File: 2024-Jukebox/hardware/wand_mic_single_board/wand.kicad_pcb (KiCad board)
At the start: 4 copper layers, 17.5 x 39 mm, 50 parts, among them J1 USB_C_Receptacle_USB2.0, J10 Conn_01x03, J4 Conn_01x02, J6 Conn_01x01, J9 Conn_01x02, Q1 MUN5214DW1T1G, Q3 CJ3139K, U1 CP2104, U2 ESP32-PICO-D4, U3 ICM-20948, U4 TP4065-4.2V, U5 TLV76718DRVx, U6 LY68L6400SLIT, U7 PCA9306, U9 TLV76733DRVx

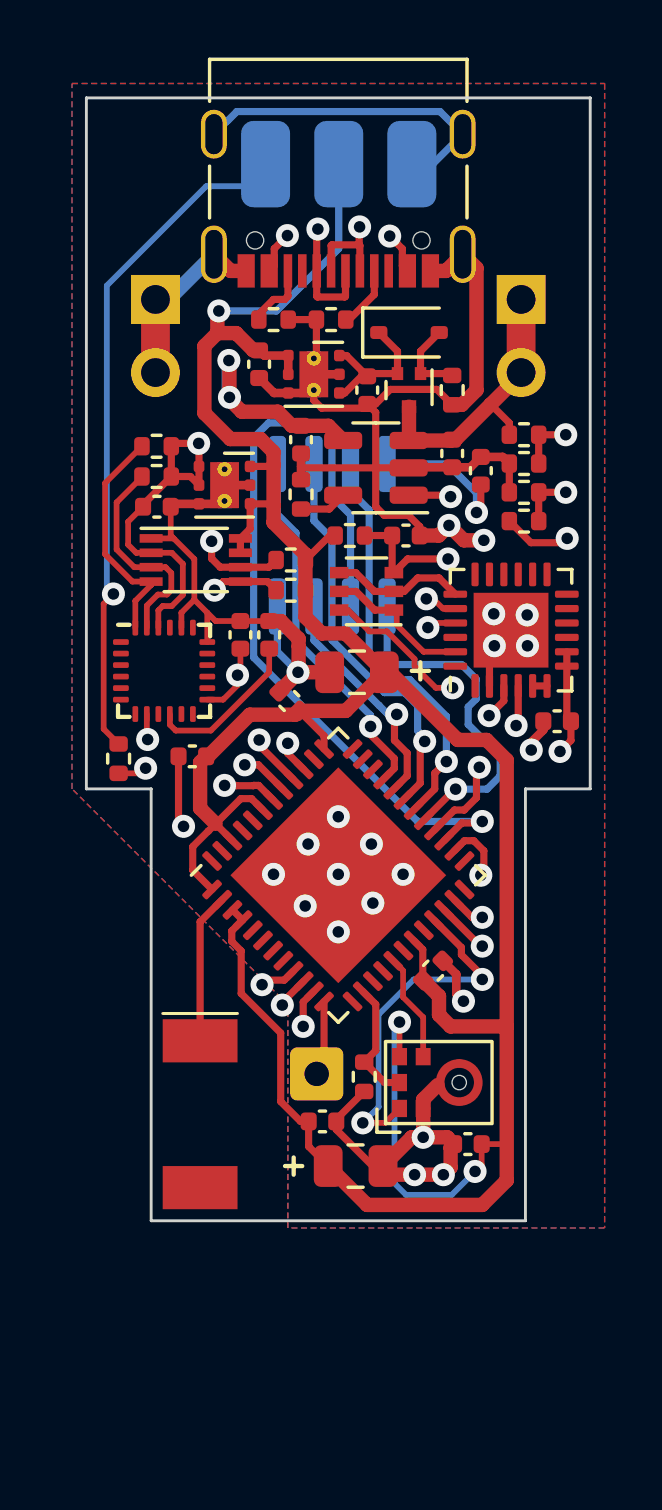
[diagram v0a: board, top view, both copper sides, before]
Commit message: Updated wand PCBs
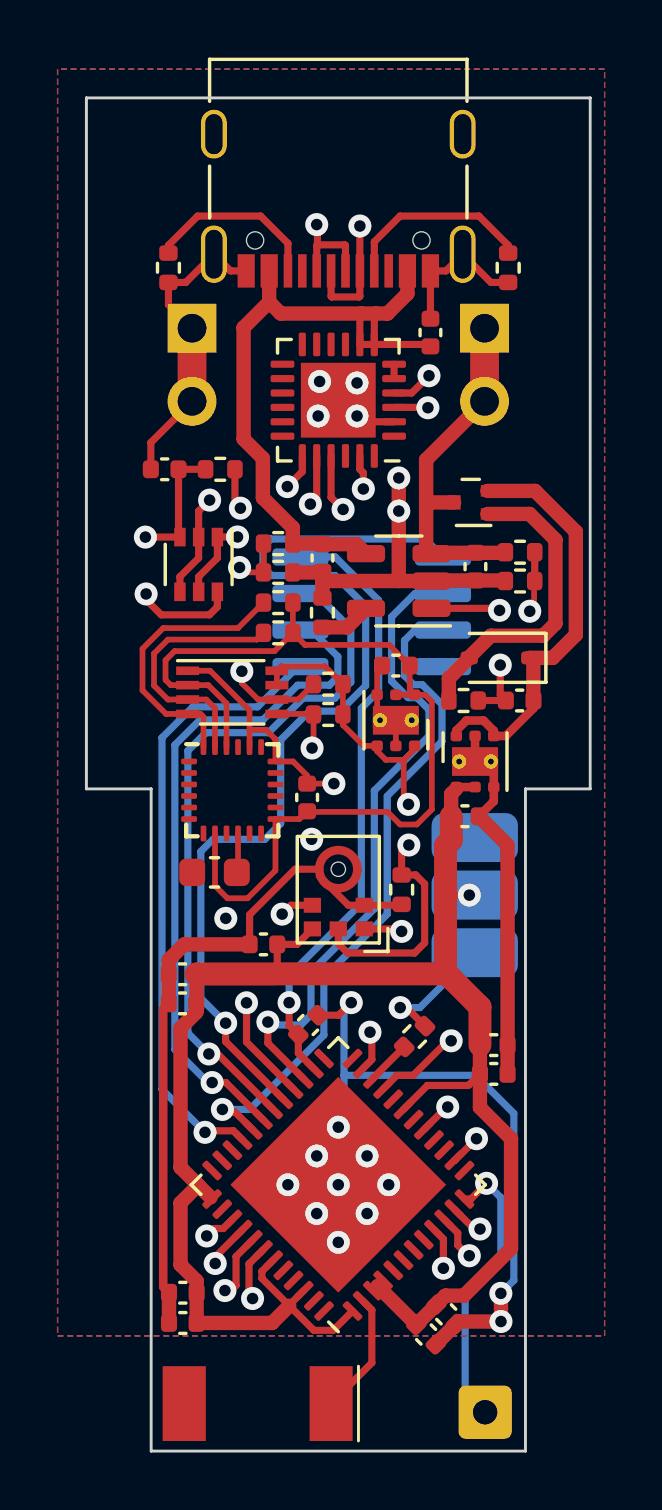
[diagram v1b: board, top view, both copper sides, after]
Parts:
- removed C14, C15: 47u, Capacitor_SMD:C_0805_2012Metric
- added C22: 10u, Capacitor_SMD:C_0402_1005Metric, F.Cu at (3.34, 30.4)
- added C23: 10u, Capacitor_SMD:C_0402_1005Metric, F.Cu at (3.35, 41.5)
- added C24: 10u, Capacitor_SMD:C_0402_1005Metric, F.Cu at (14.2, 32.9)
- added C25: 10u, Capacitor_SMD:C_0402_1005Metric, F.Cu at (12.5, 42.2)
- C9: footprint Capacitor_SMD:C_0402_1005Metric -> Capacitor_SMD:C_0603_1608Metric
- moved J10 28.3 mm to (13.5, 29.7), turned to 0 degrees
- moved C16 22.5 mm to (11.8, 43.0), turned to -45 degrees
- moved C5 20.2 mm to (7.70, 32.2), turned to 45 degrees
- moved C11 17.3 mm to (13.2, 24.9), turned to 0 degrees
- moved U9 14.6 mm to (13.5, 23.1), turned to 90 degrees
- moved C3 14.2 mm to (11.9, 8.15), turned to 90 degrees
- moved R11 14.1 mm to (11.4, 32.6), turned to -135 degrees
- moved J6 13.1 mm to (13.8, 45.6)
- moved C10 12.0 mm to (15.1, 20.9), turned to 180 degrees
- moved D1 11.7 mm to (14.3, 19.4), turned to 180 degrees
- moved R18 10.8 mm to (13.1, 20.9), turned to 180 degrees
- moved U2 10.8 mm to (8.75, 37.8), turned to 135 degrees
- moved AE1 10.2 mm to (5.95, 45.4), turned to 180 degrees
- moved U5 10.1 mm to (10.8, 21.6), turned to -90 degrees
- moved U1 9.99 mm to (8.75, 10.5), turned to 180 degrees
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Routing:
- net GND: track 94.0 -> 146.8 mm
- net VBUS: track 49.5 -> 23.9 mm, vias 6 -> 0
- net RXD: track 11.7 -> 33.3 mm
- net GPIO10: track 12.4 -> 33.8 mm
- net TXD: track 14.3 -> 35.0 mm
- net Net-(J10-Pin_1): track 23.6 -> 4.51 mm
- net GPIO2: track 19.7 -> 1.56 mm, vias 2 -> 0
- net GPIO25: track 4.33 -> 21.6 mm, vias 0 -> 2
- net GPIO0: track 15.5 -> 32.6 mm
- net GPIO7: track 8.15 -> 23.5 mm
- net IMU_SCL: track 12.3 -> 27.6 mm
- net RESET: track 24.0 -> 39.2 mm
- net GPIO9: track 17.5 -> 32.2 mm
- net Net-(U1-D+): track 27.1 -> 12.6 mm
- net IMU_SDA: track 12.4 -> 26.3 mm
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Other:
- board size 17.5 x 39 mm -> 17.5 x 47 mm
- board text added: "SRAM"
